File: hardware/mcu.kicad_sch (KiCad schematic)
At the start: 28 parts, among them J5 Conn_01x02_MountingPin, J6 USB_C_Receptacle_USB2.0_14P, Q1 MMBT3904, Q2 MMBT3904, SW1 SW_Push, U1 ESP32-C3, U2 MCP2562-E-SN, Y1 40MHz

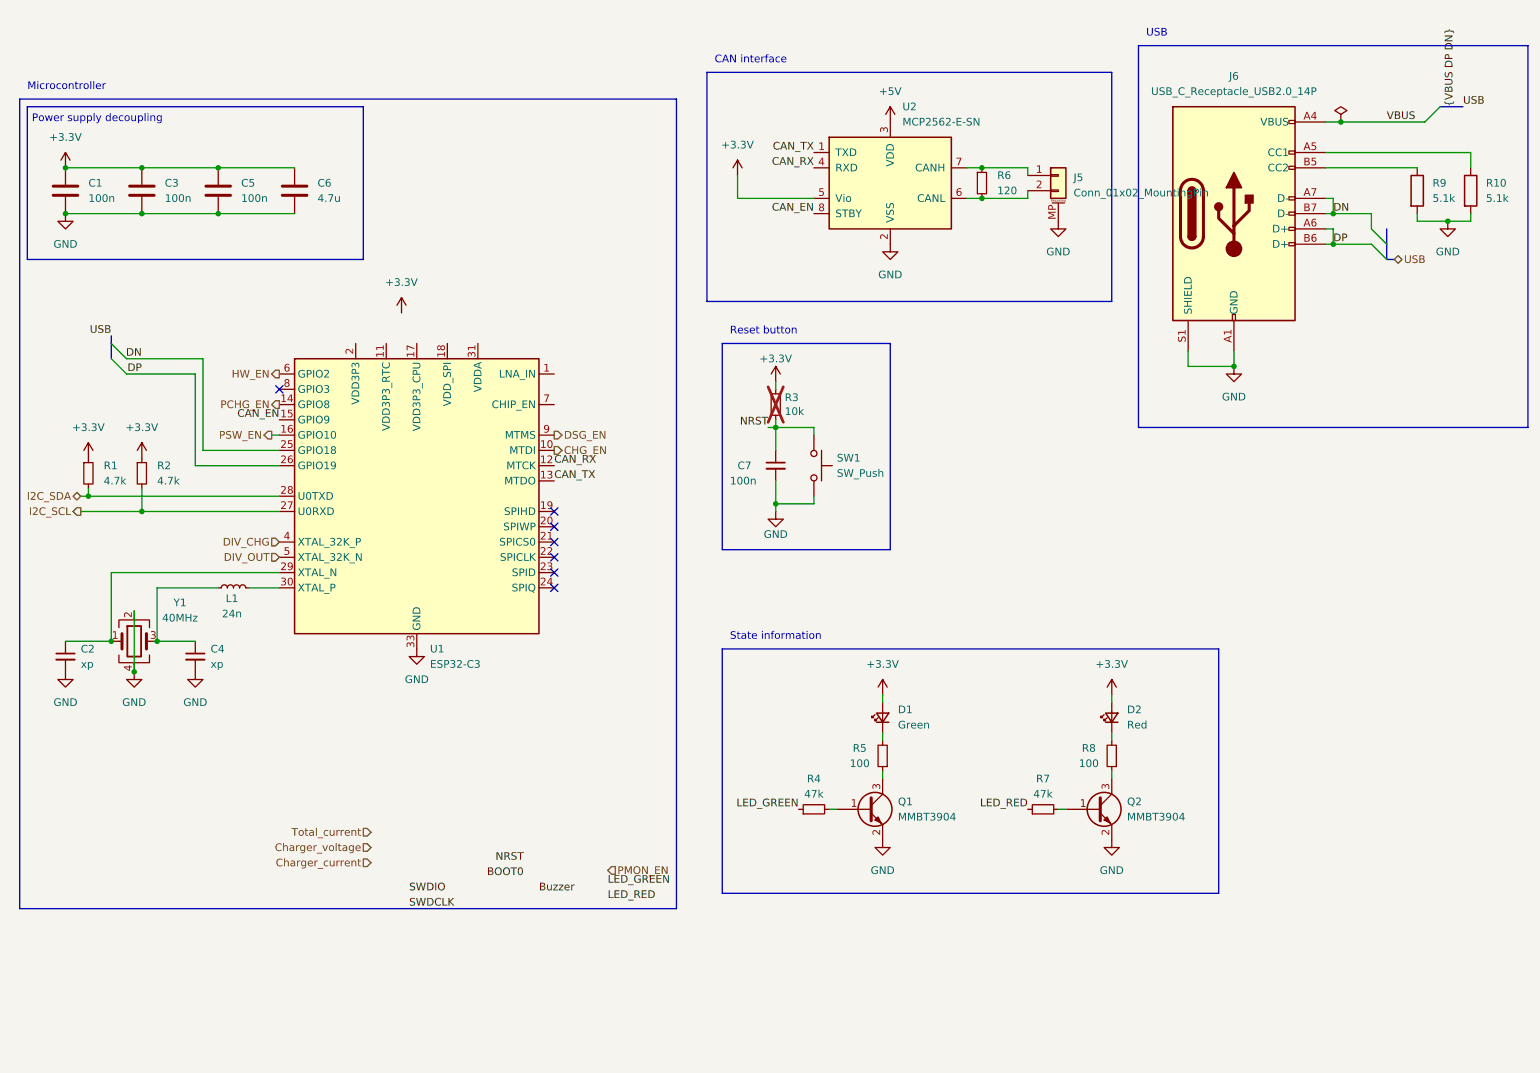
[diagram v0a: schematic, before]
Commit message: Various changes (can't remember)
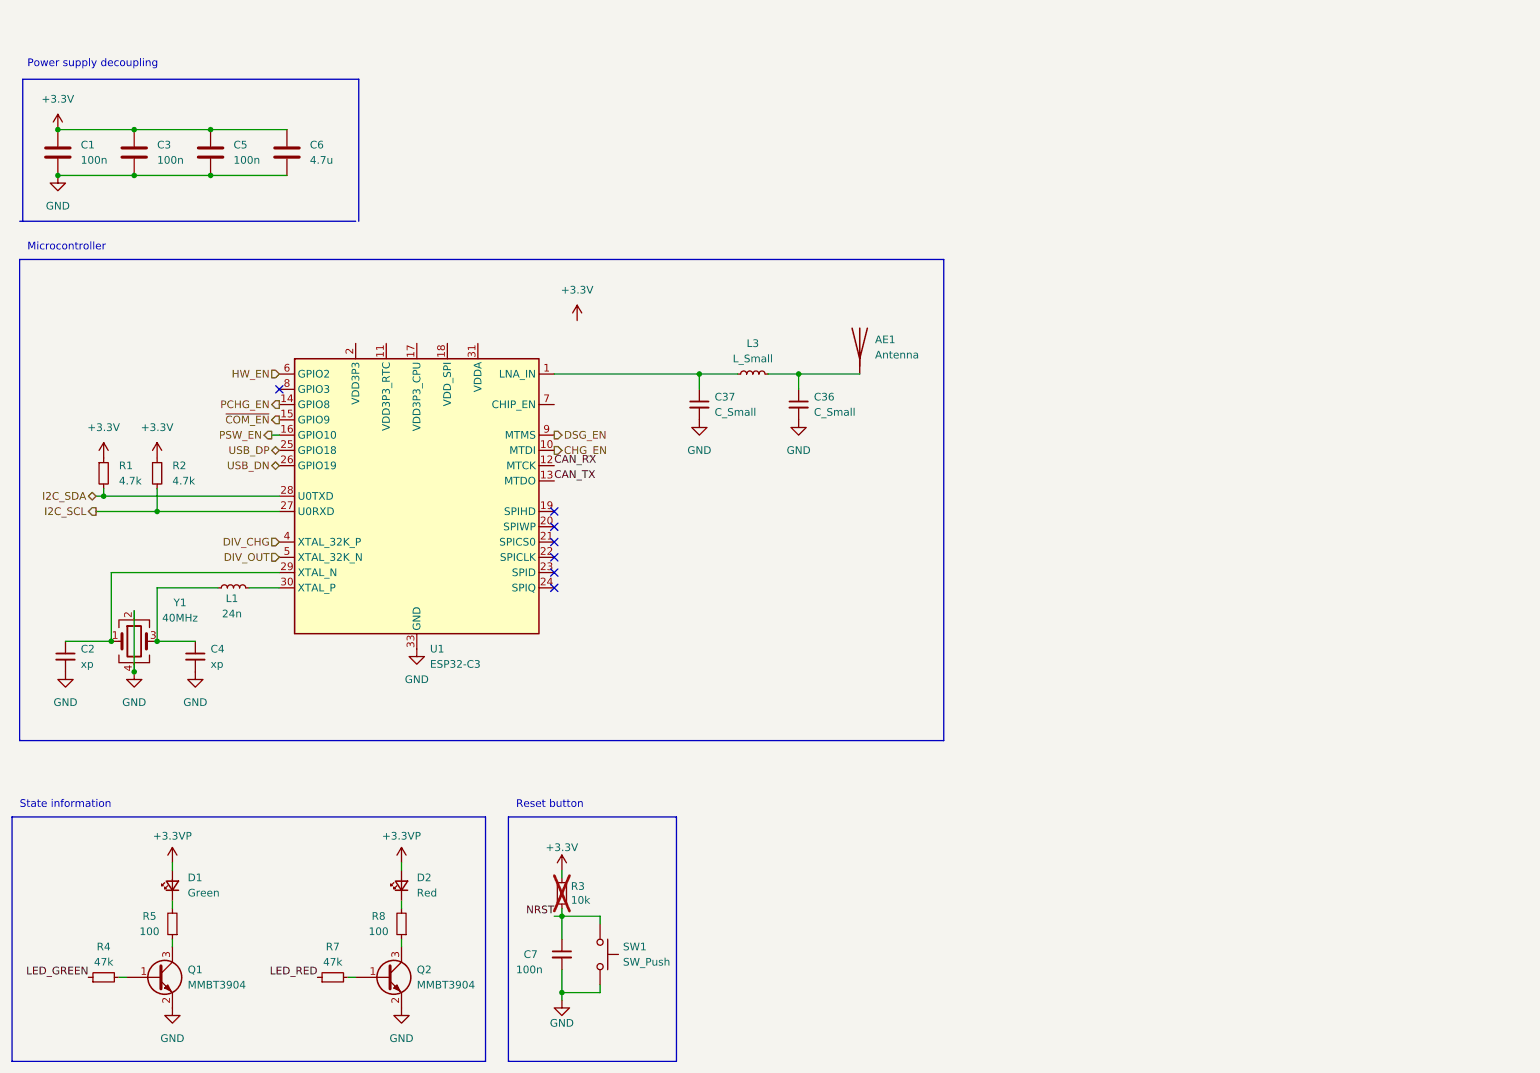
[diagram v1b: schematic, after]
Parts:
- removed J5: Conn_01x02_MountingPin, Connector_JST:JST_PH_B2B-PH-SM4-TB_1x02-1MP_P2.00mm_Vertical, symbol Connector_Generic_MountingPin:Conn_01x02_MountingPin
- removed J6: USB_C_Receptacle_USB2.0_14P, Connector_USB:USB_C_Receptacle_Palconn_UTC16-G, symbol Connector:USB_C_Receptacle_USB2.0_14P
- removed R10, R9: 5.1k, Resistor_SMD:R_0603_1608Metric, symbol Device:R
- removed R6: 120, Resistor_SMD:R_0603_1608Metric, symbol Device:R_Small
- removed U2: MCP2562-E-SN, Package_SO:SOIC-8_3.9x4.9mm_P1.27mm, symbol Interface_CAN_LIN:MCP2562-E-SN
- added AE1: Antenna, symbol Device:Antenna
- added C36, C37: C_Small, symbol Device:C_Small
- added L3: L_Small, symbol Device:L_Small
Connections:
- net +3.3V: no longer D1.2 (A), D2.2 (A)
- net GND: now also C36.2, C37.2
- net at U1.1 (LNA_IN): now also C37.1, L3.1
- net CAN_EN renamed ~{COM_EN}
- net DN renamed USB_DP
- net DP renamed USB_DN
- new net: AE1.1 (A), C36.1, L3.2
- new net +3.3VP: D1.2 (A), D2.2 (A)
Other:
- note removed: "CAN interface"
- note removed: "USB"
- moved on the sheet: C1, C3, C5, C6, C7, D1, D2, Q1, Q2, R1, R2, R3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

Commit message: ESP32 Decoupling
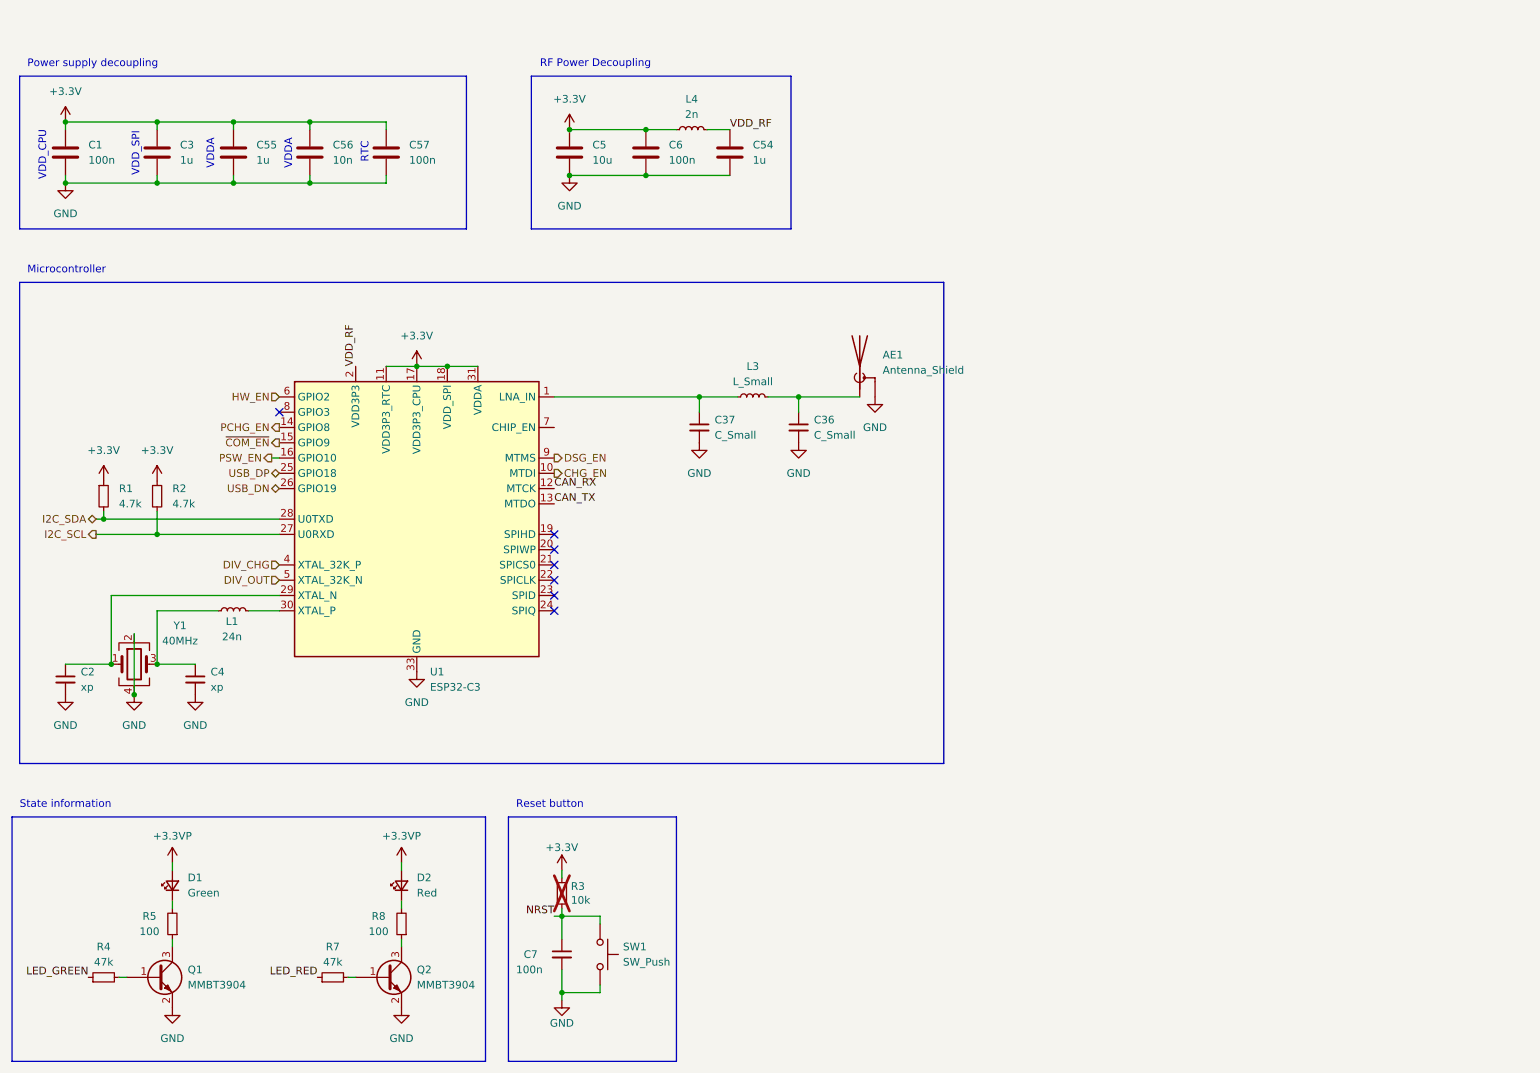
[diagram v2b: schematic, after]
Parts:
- removed AE1: Antenna, symbol Device:Antenna
- added AE1: Antenna_Shield, RF_Antenna:Texas_SWRA117D_2.4GHz_Left, symbol Device:Antenna_Shield
- added C54, C55: 1u, Capacitor_SMD:C_0402_1005Metric, symbol Device:C
- added C56: 10n, Capacitor_SMD:C_0402_1005Metric, symbol Device:C
- added C57: 100n, Capacitor_SMD:C_0402_1005Metric, symbol Device:C
- added L4: 2n, symbol Device:L_Small
- C3: value 100n -> 1u
- C5: value 100n -> 10u
- C6: value 4.7u -> 100n
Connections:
- net +3.3V: now also U1.11 (VDD3P3_RTC), U1.17 (VDD3P3_CPU), U1.18 (VDD_SPI), U1.31 (VDDA), U1.32 (VDDA), C55.1, C56.1, C57.1, L4.1
- net GND: now also AE1.2 (Shield), C54.2, C55.2, C56.2, C57.2
- net at C36.1, L3.2: now also AE1.1 (A)
- net VDD_RF: now reaches U1.2 (VDD3P3), U1.3 (VDD3P3)
- net VDD_RF: now also C54.1, L4.2
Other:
- note added: "RF Power Decoupling"
- note added: "RTC"
- note added: "VDDA"
- note added: "VDD_CPU"
- note added: "VDD_SPI"
- moved on the sheet: C1, C2, C3, C36, C37, C4, C5, C6, L1, L3, R1, R2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
